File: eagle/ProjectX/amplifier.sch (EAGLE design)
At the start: 8 parts, among them U1 TC4427COA, U2 TC4427COA

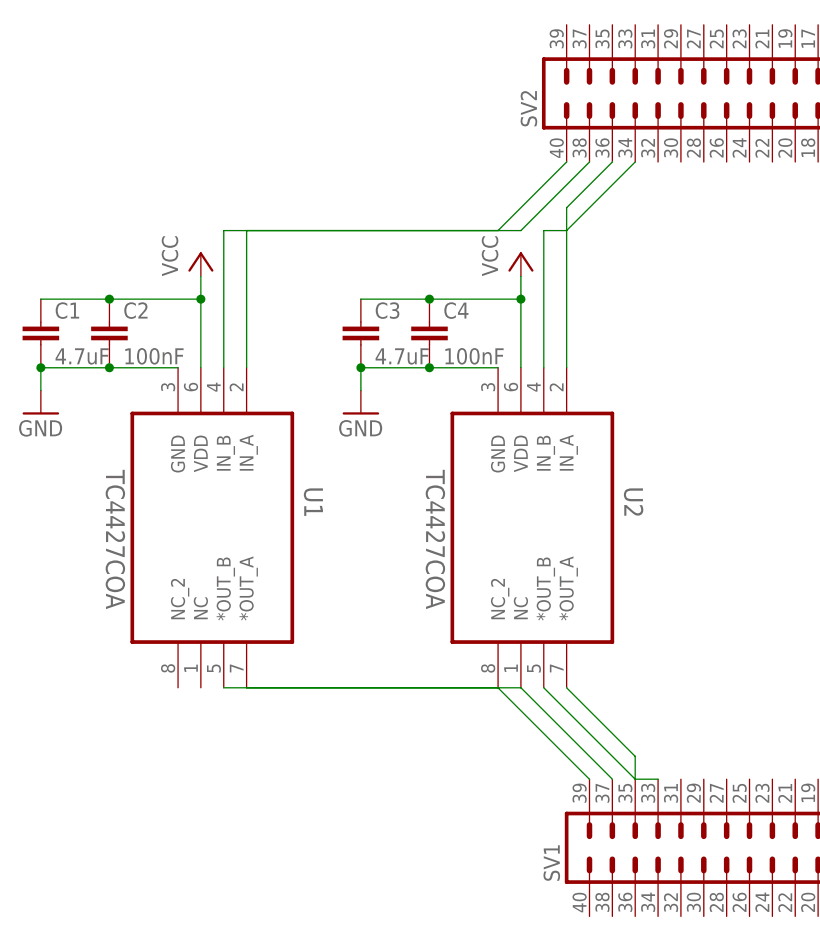
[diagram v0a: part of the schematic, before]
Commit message: Some work on the final design
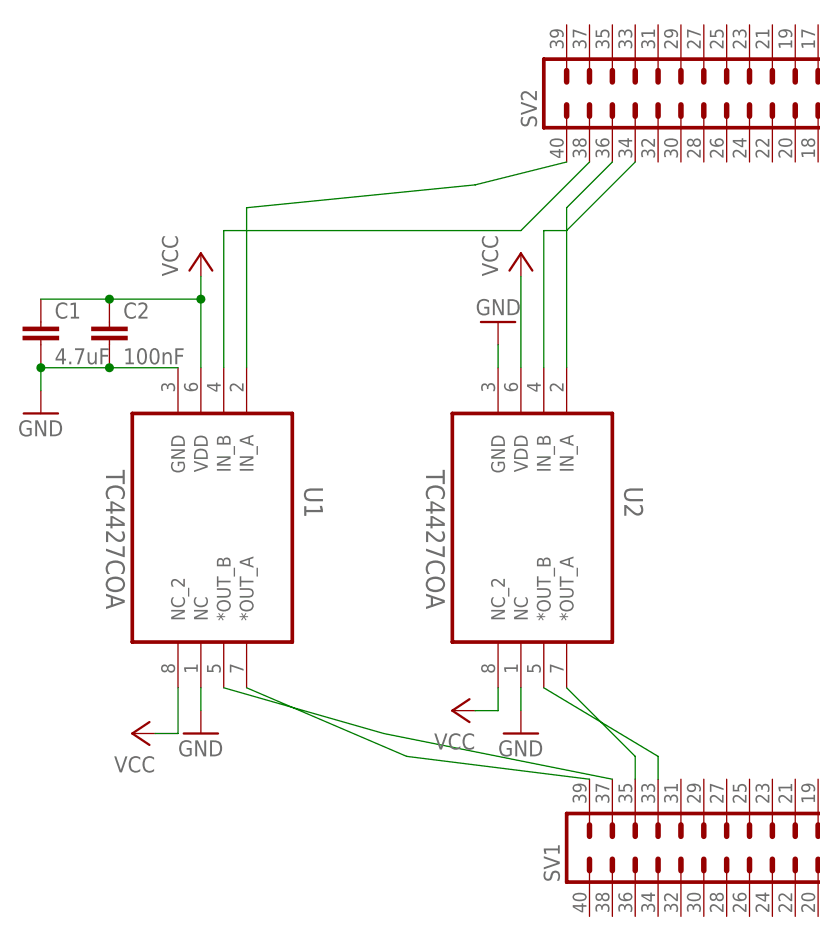
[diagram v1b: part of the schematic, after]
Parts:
- removed C3: 4.7uF, rcl:C-EUC0805
- removed C4: 100nF, rcl:C-EUC0805
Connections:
- net GND: now also U1.NC, U2.NC; no longer C3.2, C4.2
- net VCC: now also U1.NC_2, U2.NC_2; no longer C3.1, C4.1
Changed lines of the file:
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@@
 <?xml version="1.0" encoding="utf-8"?>
 <!DOCTYPE eagle SYSTEM "eagle.dtd">
-<eagle version="8.3.2">
+<eagle version="8.4.1">
 <drawing>
 <settings>
@@
 <part name="P+5" library="supply1" library_urn="urn:adsk.eagle:library:371" deviceset="VCC" device=""/>
 <part name="U2" library="Microchip_By_element14_Batch_1" deviceset="TC4427COA" device=""/>
-<part name="C3" library="rcl" library_urn="urn:adsk.eagle:library:334" deviceset="C-EU" device="C0805" package3d_urn="urn:adsk.eagle:package:23617/2" value="4.7uF"/>
-<part name="C4" library="rcl" library_urn="urn:adsk.eagle:library:334" deviceset="C-EU" device="C0805" package3d_urn="urn:adsk.eagle:package:23617/2" value="100nF"/>
 <part name="P+6" library="supply1" library_urn="urn:adsk.eagle:library:371" deviceset="VCC" device=""/>
 <part name="GND6" library="supply1" library_urn="urn:adsk.eagle:library:371" deviceset="GND" device=""/>
+<part name="GND7" library="supply1" library_urn="urn:adsk.eagle:library:371" deviceset="GND" device=""/>
+<part name="P+7" library="supply1" library_urn="urn:adsk.eagle:library:371" deviceset="VCC" device=""/>
+<part name="P+8" library="supply1" library_urn="urn:adsk.eagle:library:371" deviceset="VCC" device=""/>
+<part name="GND8" library="supply1" library_urn="urn:adsk.eagle:library:371" deviceset="GND" device=""/>
 </parts>
 <sheets>
@@
 <instance part="P+5" gate="VCC" x="55.88" y="111.76"/>
 <instance part="U2" gate="A" x="10.16" y="43.18" rot="R270"/>
-<instance part="C3" gate="G$1" x="-12.7" y="66.04"/>
-<instance part="C4" gate="G$1" x="-5.08" y="66.04"/>
 <instance part="P+6" gate="VCC" x="5.08" y="73.66"/>
-<instance part="GND6" gate="1" x="-12.7" y="55.88"/>
+<instance part="GND6" gate="1" x="2.54" y="66.04" rot="R180"/>
+<instance part="GND7" gate="1" x="5.08" y="20.32"/>
+<instance part="P+7" gate="VCC" x="-38.1" y="20.32" rot="R90"/>
+<instance part="P+8" gate="VCC" x="-2.54" y="22.86" rot="R90"/>
+<instance part="GND8" gate="1" x="-30.48" y="20.32"/>
 </instances>
 <busses>
@@
 <pinref part="U2" gate="A" pin="VDD"/>
 <pinref part="P+6" gate="VCC" pin="VCC"/>
-<wire x1="5.08" y1="60.96" x2="5.08" y2="68.58" width="0.1524" layer="91"/>
-<pinref part="C4" gate="G$1" pin="1"/>
-<wire x1="5.08" y1="68.58" x2="5.08" y2="71.12" width="0.1524" layer="91"/>
-<wire x1="5.08" y1="68.58" x2="-5.08" y2="68.58" width="0.1524" layer="91"/>
-<junction x="5.08" y="68.58"/>
-<pinref part="C3" gate="G$1" pin="1"/>
-<wire x1="-5.08" y1="68.58" x2="-12.7" y2="68.58" width="0.1524" layer="91"/>
-<junction x="-5.08" y="68.58"/>
+<wire x1="5.08" y1="60.96" x2="5.08" y2="71.12" width="0.1524" layer="91"/>
+</segment>
+<segment>
+<pinref part="P+8" gate="VCC" pin="VCC"/>
+<pinref part="U2" gate="A" pin="NC_2"/>
+<wire x1="0" y1="22.86" x2="2.54" y2="22.86" width="0.1524" layer="91"/>
+<wire x1="2.54" y1="22.86" x2="2.54" y2="25.4" width="0.1524" layer="91"/>
+</segment>
+<segment>
+<pinref part="P+7" gate="VCC" pin="VCC"/>
+<pinref part="U1" gate="A" pin="NC_2"/>
+<wire x1="-35.56" y1="20.32" x2="-33.02" y2="20.32" width="0.1524" layer="91"/>
+<wire x1="-33.02" y1="20.32" x2="-33.02" y2="25.4" width="0.1524" layer="91"/>
 </segment>
 </net>
@@
 <segment>
 <pinref part="U2" gate="A" pin="GND"/>
-<pinref part="C4" gate="G$1" pin="2"/>
-<wire x1="2.54" y1="60.96" x2="-5.08" y2="60.96" width="0.1524" layer="91"/>
-<pinref part="C3" gate="G$1" pin="2"/>
-<wire x1="-5.08" y1="60.96" x2="-12.7" y2="60.96" width="0.1524" layer="91"/>
-<junction x="-5.08" y="60.96"/>
+<wire x1="2.54" y1="60.96" x2="2.54" y2="63.5" width="0.1524" layer="91"/>
 <pinref part="GND6" gate="1" pin="GND"/>
-<wire x1="-12.7" y1="58.42" x2="-12.7" y2="60.96" width="0.1524" layer="91"/>
-<junction x="-12.7" y="60.96"/>
+</segment>
+<segment>
+<pinref part="U2" gate="A" pin="NC"/>
+<pinref part="GND7" gate="1" pin="GND"/>
+<wire x1="5.08" y1="25.4" x2="5.08" y2="22.86" width="0.1524" layer="91"/>
+</segment>
+<segment>
+<pinref part="U1" gate="A" pin="NC"/>
+<pinref part="GND8" gate="1" pin="GND"/>
+<wire x1="-30.48" y1="25.4" x2="-30.48" y2="22.86" width="0.1524" layer="91"/>
 </segment>
 </net>
@@
 <net name="N$5" class="0">
 <segment>
-<wire x1="-25.4" y1="76.2" x2="-25.4" y2="60.96" width="0.1524" layer="91"/>
+<wire x1="-25.4" y1="78.74" x2="-25.4" y2="60.96" width="0.1524" layer="91"/>
 <pinref part="U1" gate="A" pin="IN_A"/>
 <pinref part="SV2" gate="1" pin="40"/>
-<wire x1="-25.4" y1="76.2" x2="2.54" y2="76.2" width="0.1524" layer="91"/>
-<wire x1="2.54" y1="76.2" x2="10.16" y2="83.82" width="0.1524" layer="91"/>
+<wire x1="-25.4" y1="78.74" x2="0" y2="81.28" width="0.1524" layer="91"/>
+<wire x1="0" y1="81.28" x2="10.16" y2="83.82" width="0.1524" layer="91"/>
 </segment>
 </net>
@@
 <pinref part="SV1" gate="1" pin="33"/>
 <pinref part="U2" gate="A" pin="*OUT_B"/>
-<wire x1="20.32" y1="15.24" x2="17.78" y2="15.24" width="0.1524" layer="91"/>
-<wire x1="17.78" y1="15.24" x2="7.62" y2="25.4" width="0.1524" layer="91"/>
+<wire x1="20.32" y1="15.24" x2="20.32" y2="17.78" width="0.1524" layer="91"/>
+<wire x1="20.32" y1="17.78" x2="7.62" y2="25.4" width="0.1524" layer="91"/>
 </segment>
 </net>
@@
 <pinref part="U1" gate="A" pin="*OUT_A"/>
 <pinref part="SV1" gate="1" pin="39"/>
-<wire x1="-25.4" y1="25.4" x2="2.54" y2="25.4" width="0.1524" layer="91"/>
-<wire x1="2.54" y1="25.4" x2="12.7" y2="15.24" width="0.1524" layer="91"/>
+<wire x1="-25.4" y1="25.4" x2="-7.62" y2="17.78" width="0.1524" layer="91"/>
+<wire x1="-7.62" y1="17.78" x2="12.7" y2="15.24" width="0.1524" layer="91"/>
 </segment>
 </net>
@@
 <pinref part="U1" gate="A" pin="*OUT_B"/>
 <pinref part="SV1" gate="1" pin="37"/>
-<wire x1="-27.94" y1="25.4" x2="5.08" y2="25.4" width="0.1524" layer="91"/>
-<wire x1="5.08" y1="25.4" x2="15.24" y2="15.24" width="0.1524" layer="91"/>
-</segment>
-</net>
+<wire x1="-27.94" y1="25.4" x2="-10.16" y2="20.32" width="0.1524" layer="91"/>
+<wire x1="-10.16" y1="20.32" x2="15.24" y2="15.24" width="0.1524" layer="91"/>
+</segment>
+</net>

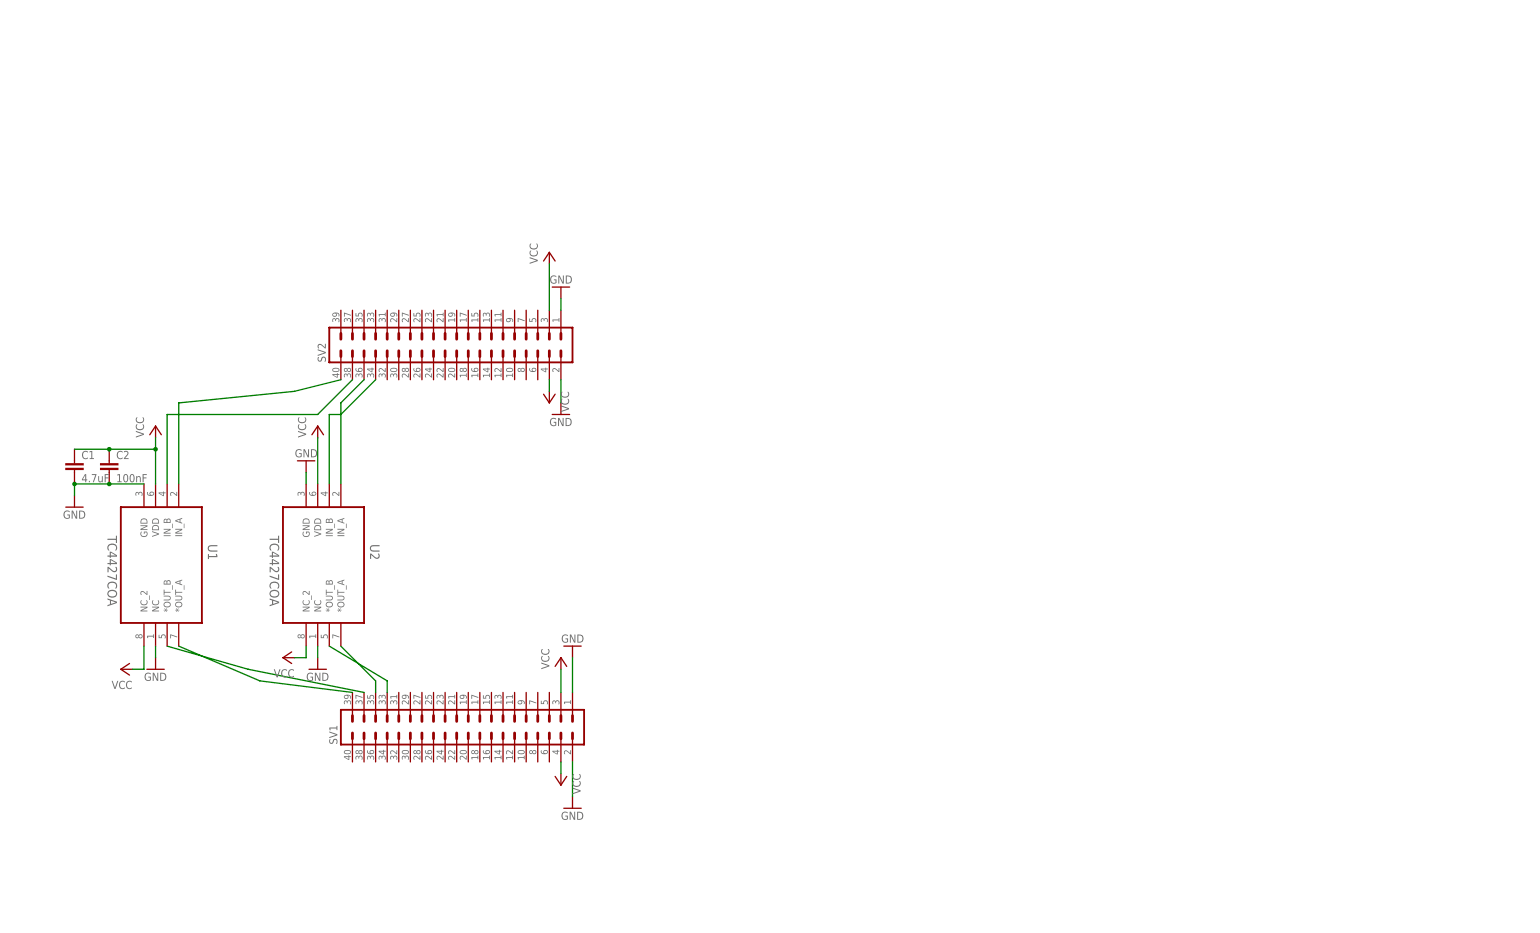
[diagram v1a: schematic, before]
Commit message: More work on the 32 bit board
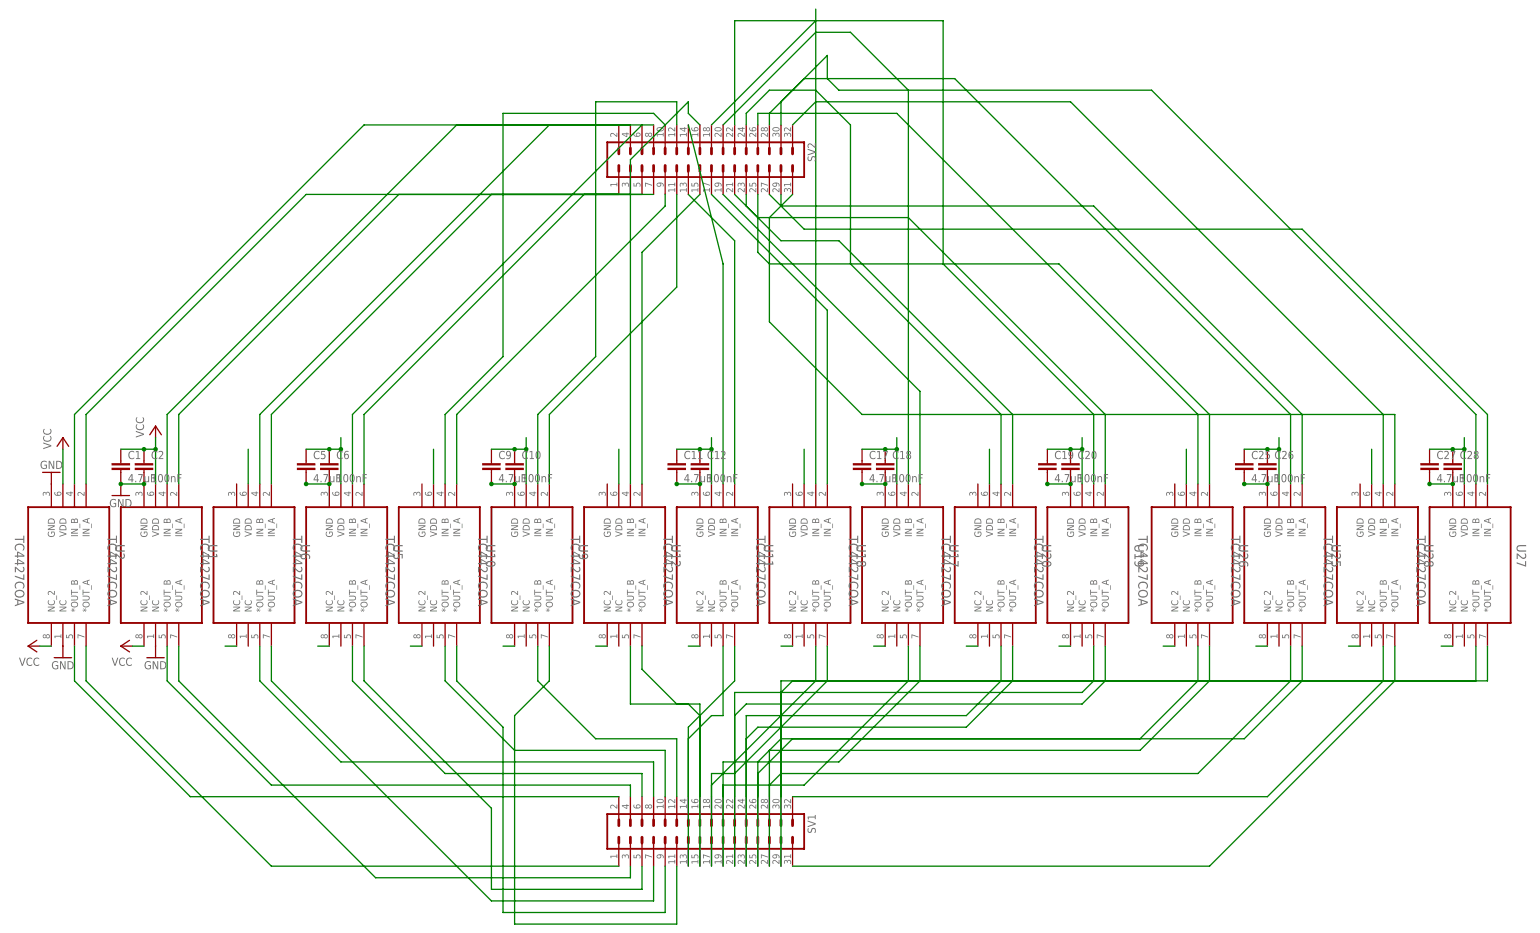
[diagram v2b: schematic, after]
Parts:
- added C10, C12, C18, C20, C26, C28, C6: 100nF, rcl:C-EUC0805
- added C11, C17, C19, C25, C27, C5, C9: 4.7uF, rcl:C-EUC0805
- added U10, U11, U12, U17, U18, U19, U20, U25, U26, U27, U28, U5, U6, U9: TC4427COA, Microchip_By_element14_Batch_1:TC4427COA
- SV1, SV2: device con-lstb:MA20-2W -> Parts:MA20-2W
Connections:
- new net N$10: SV1.1, U2.*OUT_A
- new net N$100: SV1.25, U26.*OUT_A
- new net N$101: SV1.26, U26.*OUT_B
- new net N$102: SV2.25, U26.IN_A
- new net N$103: SV1.27, U25.*OUT_A
- new net N$104: SV1.28, U25.*OUT_B
- new net N$105: SV2.30, U27.IN_B
- new net N$106: SV2.29, U27.IN_A
- new net N$107: SV2.32, U28.IN_B
- new net N$108: SV1.31, U28.*OUT_A
- new net N$109: SV1.32, U28.*OUT_B
- new net N$11: SV1.3, U1.*OUT_A
- new net N$110: SV2.31, U28.IN_A
- new net N$111: SV1.29, U27.*OUT_A
- new net N$112: SV1.30, U27.*OUT_B
- new net N$12: SV1.7, U6.*OUT_A
- new net N$13: SV1.10, U10.*OUT_B
- new net N$14: SV1.9, U10.*OUT_A
- new net N$15: SV1.11, U9.*OUT_A
- new net N$16: SV1.23, U20.*OUT_A
- new net N$17: SV2.6, U5.IN_B
- new net N$18: SV2.5, U5.IN_A
- new net N$19: SV2.8, U6.IN_B
- new net N$22: SV2.7, U6.IN_A
- new net N$23: SV1.5, U5.*OUT_A
- new net N$24: SV1.6, U5.*OUT_B
- new net N$26: SV1.15, U12.*OUT_A
- new net N$29: SV1.12, U9.*OUT_B
- new net N$33: SV2.12, U9.IN_B
- new net N$34: SV2.11, U9.IN_A
- new net N$35: SV2.10, U10.IN_B
- new net N$38: SV2.9, U10.IN_A
- new net N$41: SV2.14, U11.IN_B
- new net N$42: SV2.13, U11.IN_A
- new net N$43: SV2.16, U12.IN_B
- new net N$46: SV2.15, U12.IN_A
- new net N$47: SV1.13, U11.*OUT_A
- new net N$48: SV1.14, U11.*OUT_B
- new net N$65: SV2.20, U17.IN_B
- new net N$66: SV2.19, U17.IN_A
- new net N$67: SV2.18, U18.IN_B
- new net N$68: SV1.17, U18.*OUT_A
- new net N$69: SV1.18, U18.*OUT_B
- new net N$70: SV2.17, U18.IN_A
- new net N$71: SV1.19, U17.*OUT_A
- new net N$72: SV1.20, U17.*OUT_B
- new net N$73: SV2.22, U19.IN_B
- new net N$74: SV2.21, U19.IN_A
- new net N$75: SV2.24, U20.IN_B
- new net N$78: SV2.23, U20.IN_A
- new net N$79: SV1.21, U19.*OUT_A
- new net N$80: SV1.22, U19.*OUT_B
- new net N$9: SV1.8, U6.*OUT_B
- new net N$97: SV2.28, U25.IN_B
- new net N$98: SV2.27, U25.IN_A
- new net N$99: SV2.26, U26.IN_B
- net GND: now also C10.2, C11.2, C12.2, C17.2, C18.2, C19.2, C20.2, C25.2, C26.2, C27.2, C28.2, C5.2, C6.2, C9.2, U10.GND, U10.NC, U11.GND, U11.NC, U12.GND, U12.NC, U17.GND, U17.NC, U18.GND, U18.NC, U19.GND, U19.NC, U20.GND, U20.NC, U25.GND, U25.NC, U26.GND, U26.NC, U27.GND, U27.NC, U28.GND, U28.NC, U5.GND, U5.NC, U6.GND, U6.NC, U9.GND, U9.NC; no longer SV1.1, SV1.2, SV2.1, SV2.2
- net N$1: now also SV2.2; no longer SV2.34
- net N$2: now also SV1.2, U2.*OUT_B; no longer SV1.39, U1.*OUT_A
- net N$3: now also SV1.4; no longer SV1.37
- net N$4: now also SV2.4; no longer SV2.38
- net N$5: now also SV2.3; no longer SV2.40
- net N$6: now also SV2.1; no longer SV2.36
- net N$7: now also SV1.16, U12.*OUT_B; no longer SV1.35, U2.*OUT_A
- net N$8: now also SV1.24, U20.*OUT_B; no longer SV1.33, U2.*OUT_B
- net VCC: now also C10.1, C11.1, C12.1, C17.1, C18.1, C19.1, C20.1, C25.1, C26.1, C27.1, C28.1, C5.1, C6.1, C9.1, U10.NC_2, U10.VDD, U11.NC_2, U11.VDD, U12.NC_2, U12.VDD, U17.NC_2, U17.VDD, U18.NC_2, U18.VDD, U19.NC_2, U19.VDD, U20.NC_2, U20.VDD, U25.NC_2, U25.VDD, U26.NC_2, U26.VDD, U27.NC_2, U27.VDD, U28.NC_2, U28.VDD, U5.NC_2, U5.VDD, U6.NC_2, U6.VDD, U9.NC_2, U9.VDD; no longer SV1.3, SV1.4, SV2.3, SV2.4
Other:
- moved on the sheet: C1, C2, U2
